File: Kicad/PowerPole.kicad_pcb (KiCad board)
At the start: 2 copper layers, 198.1 x 116.8 mm, 41 parts, among them J1 Anderson powerpole, J2 Anderson powerpole, J3 Anderson powerpole, J4 Anderson powerpole, J5 Anderson powerpole, K1 896HP-1AH-C-12VDC, SW1 SW_Push

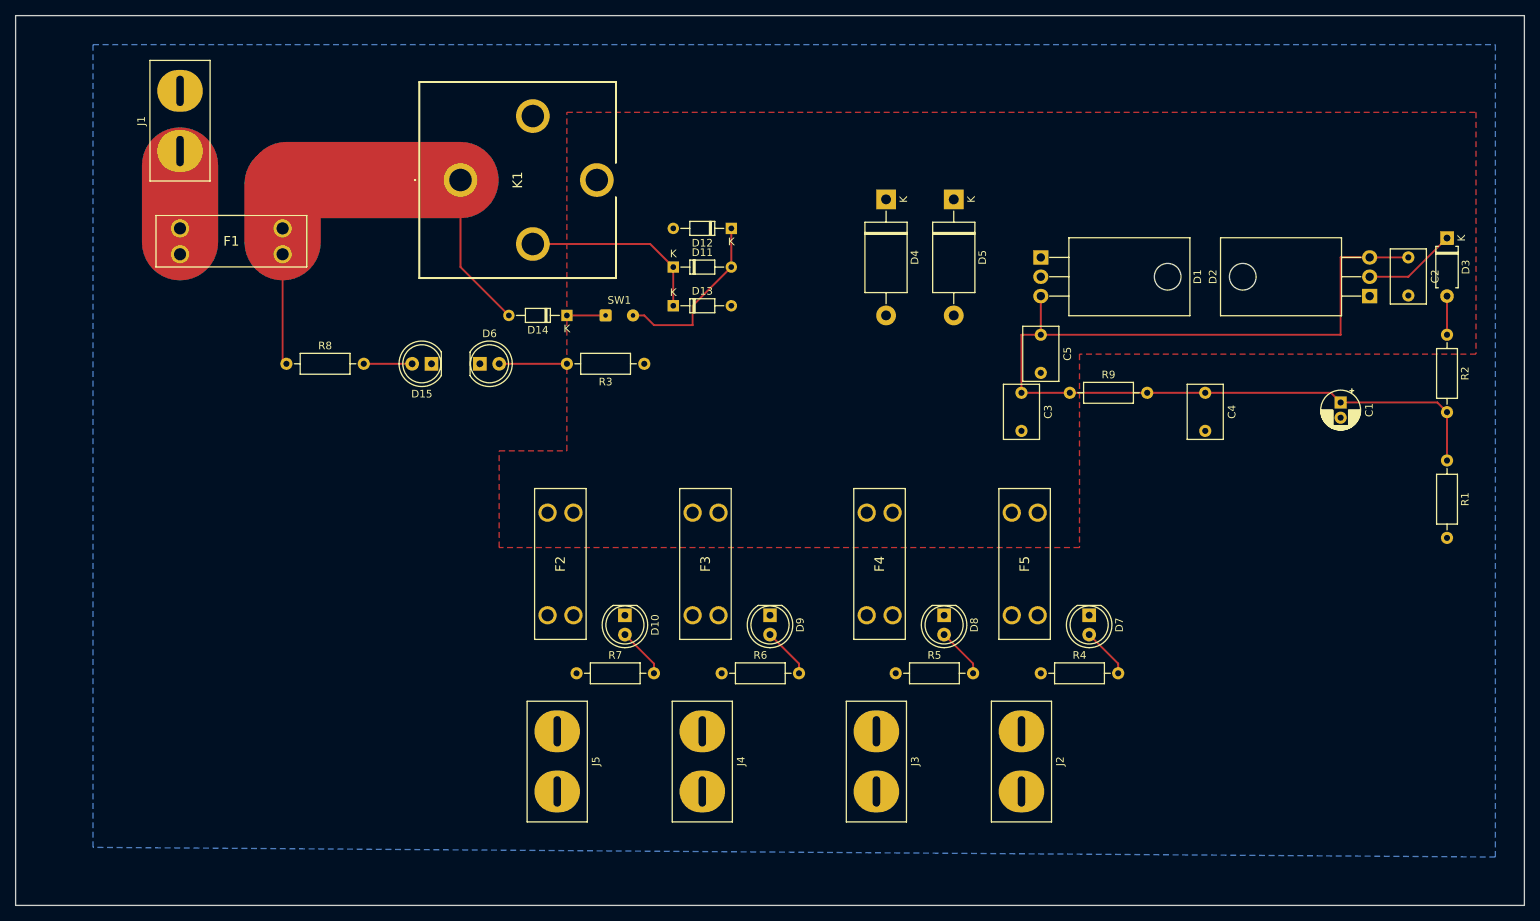
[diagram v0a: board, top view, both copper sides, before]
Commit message: PCB update
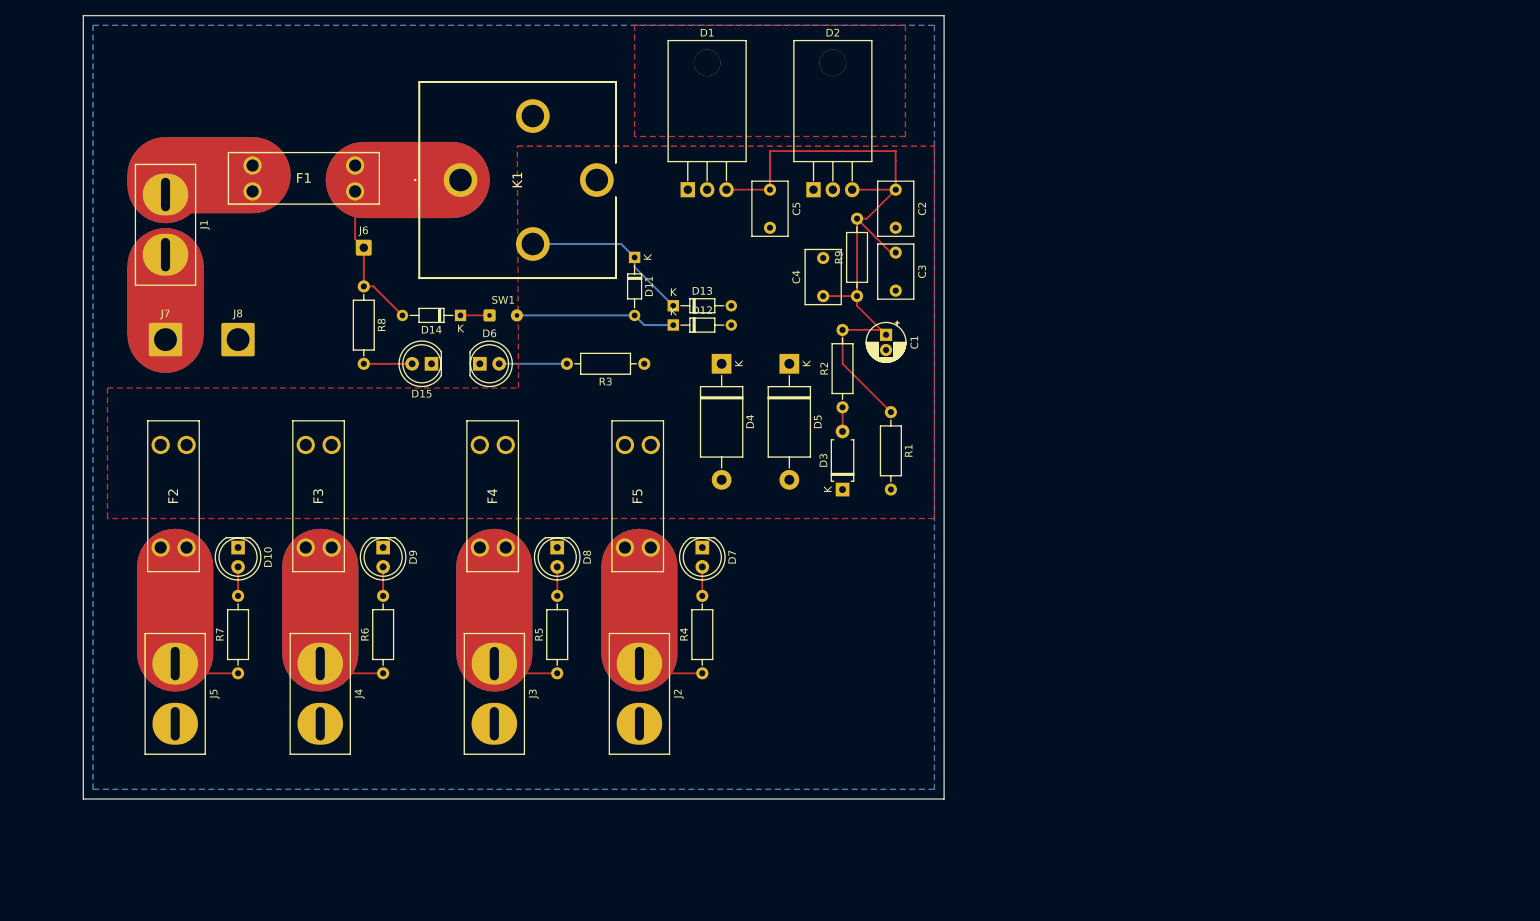
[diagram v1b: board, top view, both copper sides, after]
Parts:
- added J6: Meter +ve, Connector_Wire:SolderWire-0.5sqmm_1x01_D0.9mm_OD2.1mm, F.Cu at (124.5, 45.7)
- added J7: Meter GND, Connector_Wire:SolderWire-2.5sqmm_1x01_D2.4mm_OD4.4mm, F.Cu at (98.4, 57.8)
- added J8: Meter LOAD, Connector_Wire:SolderWire-2.5sqmm_1x01_D2.4mm_OD4.4mm, F.Cu at (108.0, 57.8)
- moved D3 86.0 mm to (187.3, 77.5), turned to 90 degrees
- moved R2 79.9 mm to (187.3, 66.7), turned to 90 degrees
- moved D2 74.3 mm to (183.5, 38.1), turned to 0 degrees
- moved R1 73.3 mm to (193.7, 67.3)
- moved C2 67.9 mm to (194.3, 38.1)
- moved C1 60.3 mm to (193.0, 57.1)
- moved C4 51.7 mm to (184.8, 52.1), turned to 90 degrees
- moved D7 51.6 mm to (168.9, 85.1)
- moved D9 51.6 mm to (127.0, 85.1)
- moved F4 51.6 mm to (139.7, 85.1)
- moved F5 51.6 mm to (158.8, 85.1)
- moved D10 51.6 mm to (108.0, 85.1)
- moved F2 51.6 mm to (97.8, 85.1)
- moved D8 51.6 mm to (149.9, 85.1)
- moved F3 51.6 mm to (116.8, 85.1)
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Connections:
- net Net-(D1-Pad2) renamed /Vout
- C1 pad 2: Net-(C1-Pad2) -> /GND
- C2 pad 2: Net-(C1-Pad2) -> /GND
- C3 pad 2: Net-(C1-Pad2) -> /GND
- C4 pad 2: Net-(C1-Pad2) -> /GND
- C5 pad 2: Net-(C1-Pad2) -> /GND
- D1 pad 1: Net-(C1-Pad2) -> /GND
- D10 pad 1: Net-(C1-Pad2) -> /GND
- D13 pad 2: Net-(C1-Pad2) -> /GND
- D15 pad 1: Net-(C1-Pad2) -> /GND
- D2 pad 1: Net-(C1-Pad2) -> /GND
- D4 pad 2: Net-(C1-Pad2) -> /GND
- D5 pad 2: Net-(C1-Pad2) -> /GND
- D6 pad 1: Net-(C1-Pad2) -> /GND
- D7 pad 1: Net-(C1-Pad2) -> /GND
- D8 pad 1: Net-(C1-Pad2) -> /GND
- D9 pad 1: Net-(C1-Pad2) -> /GND
- J1 pad 2: Net-(C1-Pad2) -> Net-(J1-Pad2)
- J2 pad 2: Net-(C1-Pad2) -> /GND
- J3 pad 2: Net-(C1-Pad2) -> /GND
- J4 pad 2: Net-(C1-Pad2) -> /GND
- J5 pad 2: Net-(C1-Pad2) -> /GND
- K1 pad 85: Net-(C1-Pad2) -> /GND
- R1 pad 2: Net-(C1-Pad2) -> /GND
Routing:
- net Net-(D14-Pad2): track 96.8 -> 42.7 mm
- net Net-(C1-Pad1): track 136.9 -> 92.3 mm
- net Net-(F4-Pad1): track 0.00 -> 32.2 mm
- net Net-(F3-Pad1): track 0.00 -> 32.2 mm
- net Net-(F5-Pad1): track 0.00 -> 32.2 mm
- net Net-(F2-Pad1): track 0.00 -> 31.5 mm
- net Net-(J1-Pad2): track 0.00 -> 18.0 mm
- net /Vout: track 12.3 -> 0.00 mm
- net Net-(F1-Pad1): track 20.2 -> 23.9 mm
- net Net-(D9-Pad2): track 6.66 -> 3.81 mm
- net Net-(D8-Pad2): track 6.66 -> 3.81 mm
- net Net-(D7-Pad2): track 6.66 -> 3.81 mm
- net Net-(D11-Pad1): track 24.8 -> 22.5 mm
- net Net-(D10-Pad2): track 6.66 -> 4.44 mm
- net Net-(D11-Pad2): track 23.2 -> 21.1 mm
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- added copper zone on F.Cu, net (none)
- added copper zone on B.Cu, net /GND
- removed copper zone on B.Cu, net Net-(C1-Pad2)
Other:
- board size 198.1 x 116.8 mm -> 113 x 102.9 mm
